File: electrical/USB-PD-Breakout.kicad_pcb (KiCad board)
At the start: 2 copper layers, 50.8 x 25.4 mm, 18 parts, among them J1 USB-C_Female, J2 CONN_02X04, J3 USB_A, J4 CONN_01X05, J5 CONN_01X02, U1 FUSB302MPX

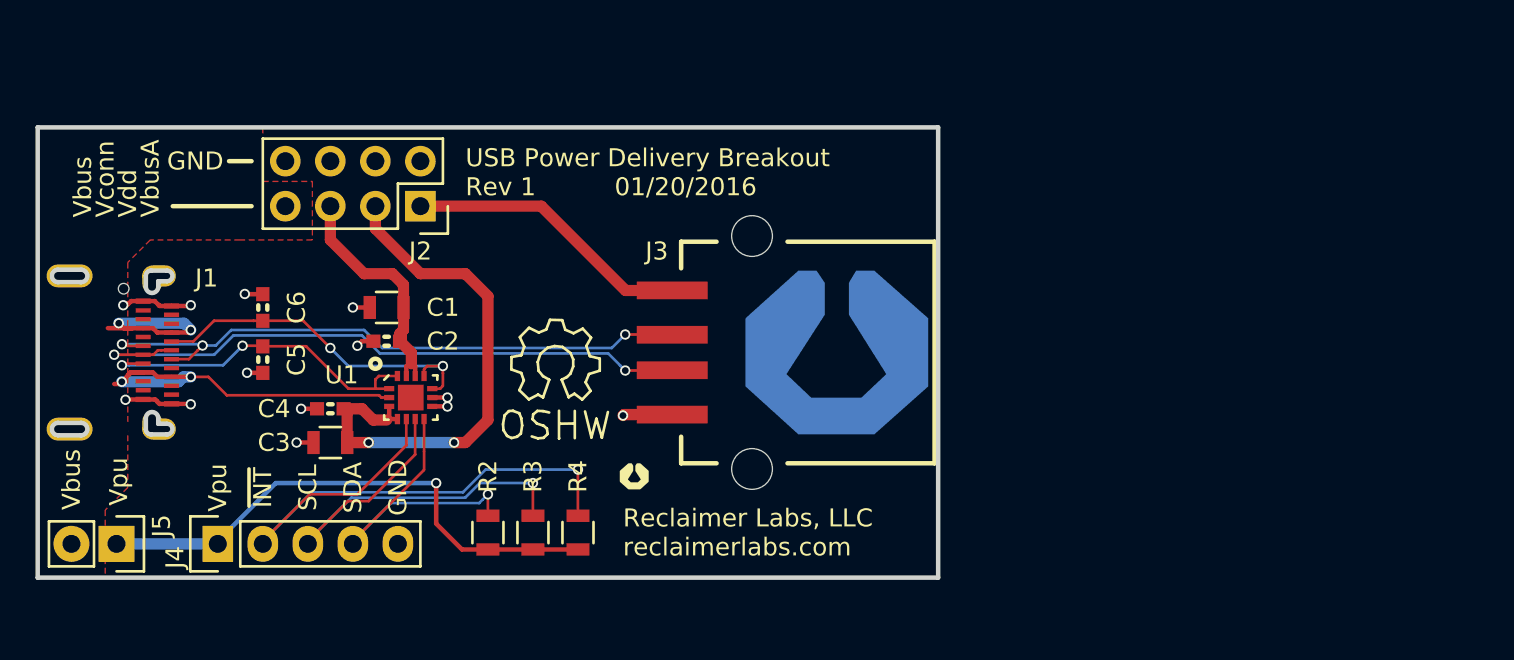
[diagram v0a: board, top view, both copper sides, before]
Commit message: Rev2 Update
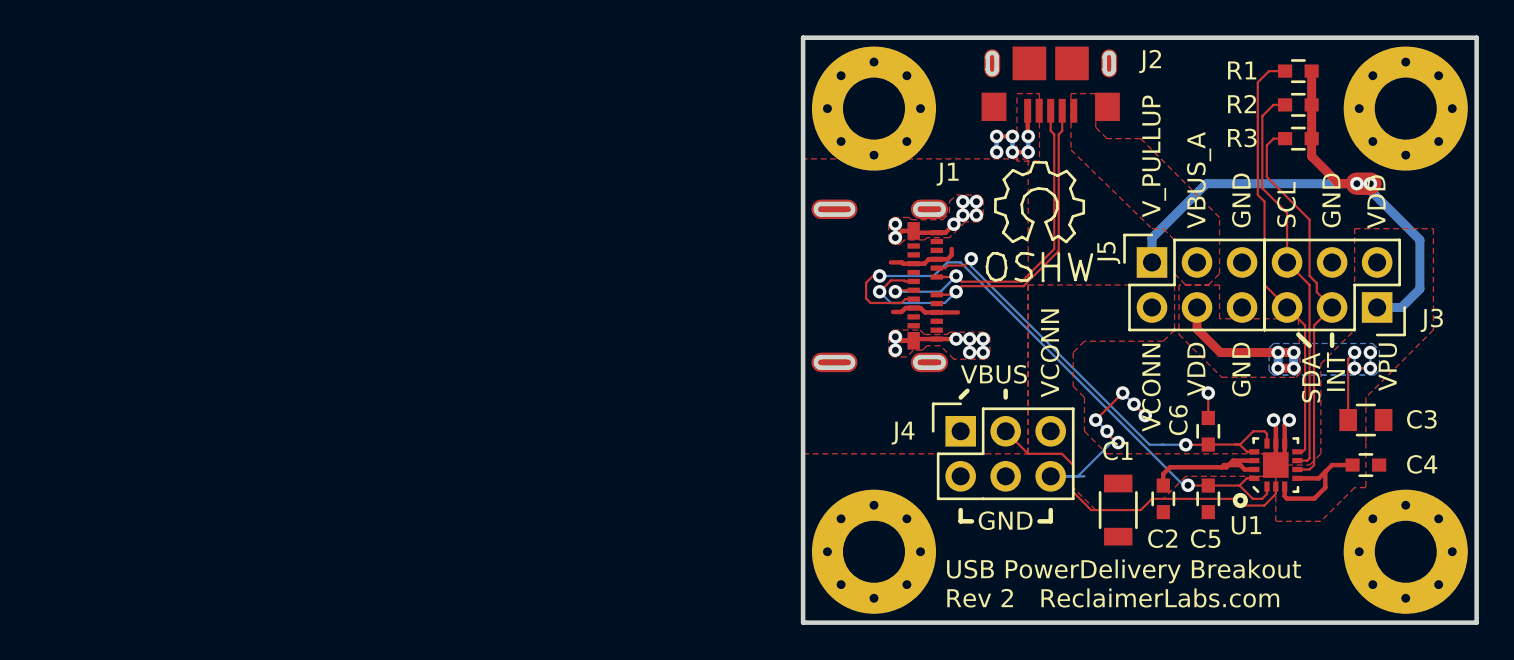
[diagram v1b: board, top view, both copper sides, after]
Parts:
- removed G***: LOGO, Jason_Libraries:Reclaimer_Labs
- removed G***: LOGO, Jason_Libraries:Reclaimer_Labs_2mm
- removed R4: 4.7k, Jason_Libraries:R_0805
- added R1: 4.7k, Capacitors_SMD:C_0603, F.Cu at (129.5, 70.5)
- added X1: MTHOLE, Reclaimer_Labs:MountingHole_3.5mm_Pad_Via, F.Cu at (105.6, 97.6)
- added X2: MTHOLE, Reclaimer_Labs:MountingHole_3.5mm_Pad_Via, F.Cu at (105.6, 72.6)
- added X3: MTHOLE, Reclaimer_Labs:MountingHole_3.5mm_Pad_Via, F.Cu at (135.6, 72.6)
- added X4: MTHOLE, Reclaimer_Labs:MountingHole_3.5mm_Pad_Via, F.Cu at (135.6, 97.6)
- C1: value 22uF -> 10uF; footprint Jason_Libraries:R_0805 -> Capacitors_SMD:C_1206
- C2, C4, C5, C6: footprint Jason_Libraries:0603_np -> Capacitors_SMD:C_0603
- C3: footprint Jason_Libraries:R_0805 -> Capacitors_SMD:C_0805
- J1: footprint Jason_Libraries:USB-C_Female_Top_Mount_Dual_SMT_RA -> Reclaimer_Labs:USB-C_Female_105450-0101
- J2: value CONN_02X04 -> USB_OTG; footprint Socket_Strips:Socket_Strip_Straight_2x04 -> Reclaimer_Labs:USB_Micro-B_10118193
- J3: value USB_A -> CONN_02X03; footprint Jason_Libraries:USB_A_Female_SMD -> Socket_Strips:Socket_Strip_Straight_2x03
- J4: value CONN_01X05 -> CONN_02X03; footprint Socket_Strips:Socket_Strip_Straight_1x05 -> Socket_Strips:Socket_Strip_Straight_2x03
- J5: value CONN_01X02 -> CONN_02X03; footprint Socket_Strips:Socket_Strip_Straight_1x02 -> Socket_Strips:Socket_Strip_Straight_2x03
- R2, R3: footprint Jason_Libraries:R_0805 -> Capacitors_SMD:C_0603
- U1: value FUSB302MPX -> FUSB302BMPX; footprint Jason_Libraries:MLP_14 -> Reclaimer_Labs:MLP_14
- moved J5 60.5 mm to (121.3, 81.3), turned to 0 degrees
- moved C4 58.5 mm to (133.3, 92.7), turned to 0 degrees
- moved C3 58.4 mm to (133.3, 90.2), turned to 0 degrees
- moved C5 53.9 mm to (124.5, 94.6)
- moved C6 53.8 mm to (124.5, 90.8)
- moved R2 51.7 mm to (129.5, 72.4), turned to 180 degrees
- moved U1 49.0 mm to (128.3, 92.7), turned to 90 degrees
- moved R3 48.6 mm to (129.5, 74.3), turned to 180 degrees
- moved C2 44.7 mm to (121.9, 94.6), turned to 270 degrees
- moved C1 42.8 mm to (119.4, 95.2), turned to 270 degrees
- moved J1 42.6 mm to (105.7, 82.6)
- moved J4 42.4 mm to (110.5, 90.8)
- moved J2 36.3 mm to (115.6, 71.0)
- moved J3 35.4 mm to (134.0, 83.8), turned to 180 degrees
- moved REF** 28.7 mm to (114.9, 78.1)
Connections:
- net /CC1 renamed /USBC_CC1
- net /CC2 renamed /USBC_CC2
- C1 pad 1: /Vconn -> VCONN
- C2 pad 1: /Vconn -> VCONN
- C3 pad 1: /Vdd -> VDD
- C4 pad 1: /Vdd -> VDD
- J1 pad A4: /Vbus -> VBUS_C
- J1 pad A6: /D+ -> /USB20_D+
- J1 pad A7: /D- -> /USB20_D-
- J1 pad A9: /Vbus -> VBUS_C
- J1 pad B4: /Vbus -> VBUS_C
- J1 pad B6: /D+ -> /USB20_D+
- J1 pad B7: /D- -> /USB20_D-
- J1 pad B9: /Vbus -> VBUS_C
- J2 pad 1: /VbusA -> VBUS_A
- J2 pad 2: GND -> /USB20_D-
- J2 pad 3: /Vdd -> /USB20_D+
- J2 pad 4: GND -> Net-(J2-Pad4)
- J2 pad 5: /Vconn -> GND
- J2 pad 6: GND -> Net-(J2-Pad6)
- J2 pad 7: /Vbus -> (no net)
- J2 pad 8: GND -> (no net)
- J3 pad 1: /VbusA -> V_PULLUP
- J3 pad 2: /D- -> VDD
- J3 pad 3: /D+ -> /~INT
- J4 pad 1: /Vpu -> VBUS_C
- J4 pad 2: /~INT -> GND
- J4 pad 3: /SCL -> VBUS_C
- J4 pad 4: /SDA -> GND
- J4 pad 5: GND -> VCONN
- J5 pad 1: /Vpu -> V_PULLUP
- J5 pad 2: /Vbus -> VCONN
- R2 pad 1: /Vpu -> V_PULLUP
- R2 pad 2: /SDA -> /SCL
- R3 pad 1: /Vpu -> V_PULLUP
- R3 pad 2: /SCL -> /~INT
- U1 pad 12: /Vconn -> VCONN
- U1 pad 13: /Vconn -> VCONN
- U1 pad 2: /Vbus -> VBUS_C
- U1 pad 3: /Vdd -> VDD
- U1 pad 4: /Vdd -> VDD
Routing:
- net (no net): track 152.4 -> 0.00 mm
- net /D+: track 36.1 -> 0.00 mm, vias 2 -> 0
- net /D-: track 35.5 -> 0.00 mm, vias 3 -> 0
- net V_PULLUP: track 0.00 -> 32.9 mm, vias 0 -> 2
- net /Vbus: track 31.3 -> 0.00 mm, vias 4 -> 0
- net /Vdd: track 30.8 -> 0.00 mm, vias 2 -> 0
- net /Vpu: track 30.6 -> 0.00 mm, vias 1 -> 0
- net VBUS_C: track 0.00 -> 26.9 mm
- net VDD: track 0.00 -> 24.0 mm, vias 0 -> 8
- net /USB20_D-: track 0.00 -> 22.9 mm, vias 0 -> 2
- net GND: track 18.1 -> 40.9 mm, vias 13 -> 29
- net /USB20_D+: track 0.00 -> 20.7 mm, vias 0 -> 2
- net /VbusA: track 16.2 -> 0.00 mm
- net /USBC_CC2: track 19.6 -> 33.9 mm
- net /Vconn: track 13.6 -> 0.00 mm
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- added copper zone on F.Cu, net VBUS_A
- added copper zone on F.Cu, net VBUS_C
- added copper zone on F.Cu, net VCONN
- added copper zone on B.Cu, net VDD
- added copper zone on F.Cu, net VDD
- removed copper zone on F.Cu, net /Vbus
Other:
- board size 50.8 x 25.4 mm -> 38 x 33 mm
- net class Default: clearance 0.1524 -> 0.126746; trace_width 0.1524 -> 0.127; via_dia 0.5842 -> 0.762
- rule trace_clearance: 0.1524 -> 0.126746
- rule trace_min: 0.1524 -> 0.12446
- rule via_min_drill: 0.254 -> 0.3302
- rule via_min_size: 0.508 -> 0.762
- board text added: "INT"
- board text added: "USB PowerDelivery Breakout Rev 2 ReclaimerLabs.com"
- board text added: "VBUS"
- board text added: "VBUS_A"
- board text added: "VCONN"
- board text added: "VDD"
- board text added: "VPU"
- board text added: "V_PULLUP"
- board text removed: "Reclaimer Labs, LLC reclaimerlabs.com"
- board text removed: "USB Power Delivery Breakout Rev 1 01/20/2016"
- board text removed: "Vbus"
- board text removed: "VbusA"
- board text removed: "Vconn"
- board text removed: "Vdd"
- board text removed: "Vpu"
- board text removed: "~INT"
